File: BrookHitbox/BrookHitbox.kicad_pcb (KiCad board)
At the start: 2 copper layers, 16 parts

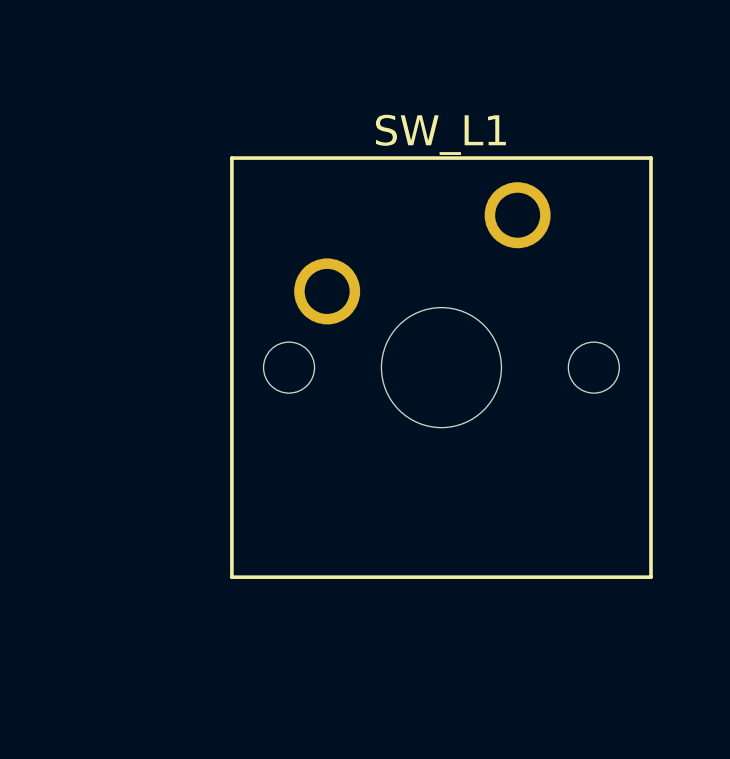
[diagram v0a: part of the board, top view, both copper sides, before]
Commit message: update pcb layout
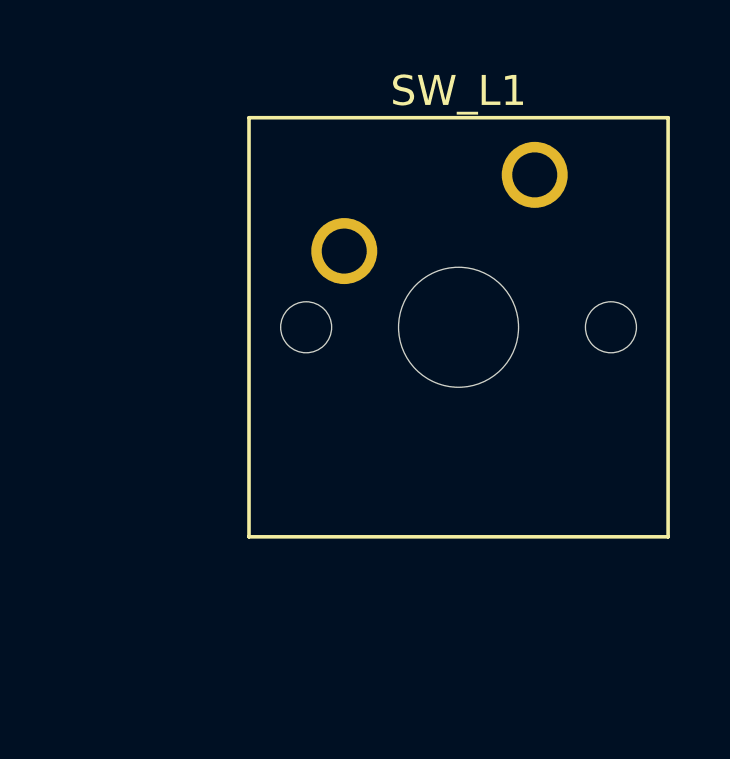
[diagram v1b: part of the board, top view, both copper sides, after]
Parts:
- moved SW_L1 1.46 mm to (276.2, 31.5)
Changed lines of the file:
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@@
         (effects (font (size 1 1) (thickness 0.15)))
     )
-    (fp_text value "~" (at -2.54 12.954) (layer "F.Fab")
+    (fp_text value "~" (at -2.54 12.954) (layer "F.Fab") hide
         (effects (font (size 1 1) (thickness 0.15)))
     )
@@
         (effects (font (size 1 1) (thickness 0.15)))
     )
-    (fp_text value "~" (at -2.54 12.954) (layer "F.Fab")
+    (fp_text value "~" (at -2.54 12.954) (layer "F.Fab") hide
         (effects (font (size 1 1) (thickness 0.15)))
     )
@@
         (effects (font (size 1 1) (thickness 0.15)))
     )
-    (fp_text value "~" (at -2.54 12.954) (layer "F.Fab")
+    (fp_text value "~" (at -2.54 12.954) (layer "F.Fab") hide
         (effects (font (size 1 1) (thickness 0.15)))
     )
@@
         (effects (font (size 1 1) (thickness 0.15)))
     )
-    (fp_text value "~" (at -2.54 12.954) (layer "F.Fab")
+    (fp_text value "~" (at -2.54 12.954) (layer "F.Fab") hide
         (effects (font (size 1 1) (thickness 0.15)))
     )
@@
         (effects (font (size 1 1) (thickness 0.15)))
     )
-    (fp_text value "~" (at -2.54 12.954) (layer "F.Fab")
+    (fp_text value "~" (at -2.54 12.954) (layer "F.Fab") hide
         (effects (font (size 1 1) (thickness 0.15)))
     )
@@
         (effects (font (size 1 1) (thickness 0.15)))
     )
-    (fp_text value "~" (at -2.54 12.954) (layer "F.Fab")
+    (fp_text value "~" (at -2.54 12.954) (layer "F.Fab") hide
         (effects (font (size 1 1) (thickness 0.15)))
     )
@@
         (effects (font (size 1 1) (thickness 0.15)))
     )
-    (fp_text value "~" (at -2.54 12.954) (layer "F.Fab")
+    (fp_text value "~" (at -2.54 12.954) (layer "F.Fab") hide
         (effects (font (size 1 1) (thickness 0.15)))
     )
@@
         (effects (font (size 1 1) (thickness 0.15)))
     )
-    (fp_text value "~" (at -2.54 12.954) (layer "F.Fab")
+    (fp_text value "~" (at -2.54 12.954) (layer "F.Fab") hide
         (effects (font (size 1 1) (thickness 0.15)))
     )
@@
         (effects (font (size 1 1) (thickness 0.15)))
     )
-    (fp_text value "~" (at -2.54 12.954) (layer "F.Fab")
+    (fp_text value "~" (at -2.54 12.954) (layer "F.Fab") hide
         (effects (font (size 1 1) (thickness 0.15)))
     )
@@
         (effects (font (size 1 1) (thickness 0.15)))
     )
-    (fp_text value "~" (at -2.54 12.954) (layer "F.Fab")
+    (fp_text value "~" (at -2.54 12.954) (layer "F.Fab") hide
         (effects (font (size 1 1) (thickness 0.15)))
     )
@@
         (effects (font (size 1 1) (thickness 0.15)))
     )
-    (fp_text value "~" (at -2.54 12.954) (layer "F.Fab")
+    (fp_text value "~" (at -2.54 12.954) (layer "F.Fab") hide
         (effects (font (size 1 1) (thickness 0.15)))
     )
@@
         (effects (font (size 1 1) (thickness 0.15)))
     )
-    (fp_text value "~" (at -2.54 12.954) (layer "F.Fab")
+    (fp_text value "~" (at -2.54 12.954) (layer "F.Fab") hide
         (effects (font (size 1 1) (thickness 0.15)))
     )
@@
         (effects (font (size 1 1) (thickness 0.15)))
     )
-    (fp_text value "~" (at -2.54 12.954) (layer "F.Fab")
+    (fp_text value "~" (at -2.54 12.954) (layer "F.Fab") hide
         (effects (font (size 1 1) (thickness 0.15)))
     )
@@
         (effects (font (size 1 1) (thickness 0.15)))
     )
-    (fp_text value "~" (at 0 -2.25 90) (layer "F.Fab")
+    (fp_text value "~" (at -2.714 -2.986 90) (layer "F.Fab") hide
         (effects (font (size 1 1) (thickness 0.15)))
     )
@@
   )
   (footprint "Button_Switch_Keyboard:SW_Cherry_MX_1.00u_PCB" (layer "F.Cu")
-    (at 275.664 32.82)
+    (at 276.234 31.475)
     (descr "Cherry MX keyswitch, 1.00u, PCB mount, http://cherryamericas.com/wp-content/uploads/2014/12/mx_cat.pdf")
     (tags "Cherry MX keyswitch 1.00u PCB")
@@
         (effects (font (size 1 1) (thickness 0.15)))
     )
-    (fp_text value "~" (at -2.54 12.954) (layer "F.Fab")
+    (fp_text value "~" (at -2.54 12.954) (layer "F.Fab") hide
         (effects (font (size 1 1) (thickness 0.15)))
     )
@@
         (effects (font (size 1 1) (thickness 0.15)))
     )
-    (fp_text value "~" (at -2.54 12.954) (layer "F.Fab")
-        (effects (font (size 1 1) (thickness 0.15)))
-    )
+    (fp_text value "~" (at -2.54 12.954) (layer "F.Fab") hide
+        (effects (font (size 1 1) (thickness 0.15)))
+    )
